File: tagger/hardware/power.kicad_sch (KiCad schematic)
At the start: 34 parts, among them J6 CHARGER, P1 USB, U12 TPS62A02DRL, U6 MAX77757JEFG420+T

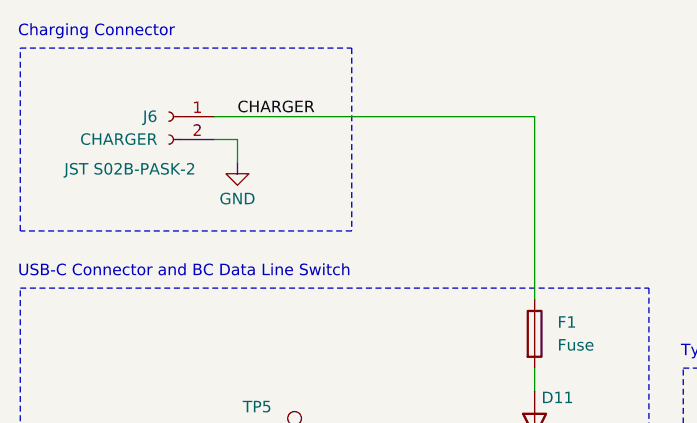
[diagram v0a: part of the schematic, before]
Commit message: chore(tagger): schematic reorganization
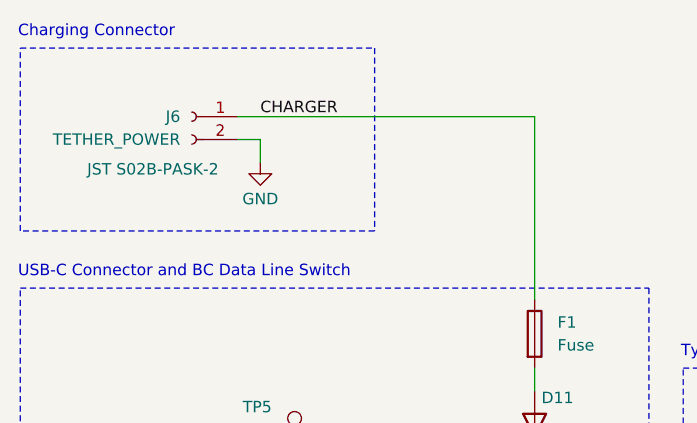
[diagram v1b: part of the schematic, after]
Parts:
- J6: value CHARGER -> TETHER_POWER
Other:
- moved on the sheet: J6
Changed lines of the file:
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@@
 	(rectangle
 		(start 17.78 20.32)
-		(end 54.61 40.64)
+		(end 57.15 40.64)
 		(stroke
 			(width 0)
@@
 	(wire
 		(pts
-			(xy 41.91 30.48) (xy 41.91 33.02)
+			(xy 44.45 30.48) (xy 44.45 33.02)
 		)
 		(stroke
@@
 	(wire
 		(pts
-			(xy 39.37 30.48) (xy 41.91 30.48)
+			(xy 41.91 30.48) (xy 44.45 30.48)
 		)
 		(stroke
@@
 	(wire
 		(pts
-			(xy 39.37 27.94) (xy 74.93 27.94)
+			(xy 41.91 27.94) (xy 74.93 27.94)
 		)
 		(stroke
@@
 	)
 	(label "CHARGER"
-		(at 41.91 27.94 0)
+		(at 44.45 27.94 0)
 		(effects
 			(font
@@
 	(symbol
 		(lib_id "Connector:Conn_01x02_Socket")
-		(at 34.29 27.94 0)
+		(at 36.83 27.94 0)
 		(mirror y)
 		(unit 1)
@@
 		(dnp no)
 		(property "Reference" "J6"
-			(at 33.02 27.9399 0)
+			(at 35.56 27.9399 0)
 			(effects
 				(font
@@
 			)
 		)
-		(property "Value" "CHARGER"
-			(at 33.02 30.4799 0)
+		(property "Value" "TETHER_POWER"
+			(at 35.56 30.4799 0)
 			(effects
 				(font
@@
 		)
 		(property "Footprint" ""
-			(at 34.29 27.94 0)
+			(at 36.83 27.94 0)
 			(effects
 				(font
@@
 		)
 		(property "Datasheet" "~"
-			(at 34.29 27.94 0)
+			(at 36.83 27.94 0)
 			(effects
 				(font
@@
 		)
 		(property "Description" "Generic connector, single row, 01x02, script generated"
-			(at 34.29 27.94 0)
+			(at 36.83 27.94 0)
 			(effects
 				(font
@@
 		)
 		(property "Conn" "JST S02B-PASK-2"
-			(at 29.972 33.782 0)
+			(at 32.512 33.782 0)
 			(effects
 				(font
@@
 	(symbol
 		(lib_id "power:GND")
-		(at 41.91 33.02 0)
+		(at 44.45 33.02 0)
 		(unit 1)
 		(exclude_from_sim no)
@@
 		(dnp no)
 		(property "Reference" "#PWR016"
-			(at 41.91 39.37 0)
+			(at 44.45 39.37 0)
 			(effects
 				(font
@@
 		)
 		(property "Value" "GND"
-			(at 41.91 37.084 0)
+			(at 44.45 37.084 0)
 			(effects
 				(font
@@
 		)
 		(property "Footprint" ""
-			(at 41.91 33.02 0)
+			(at 44.45 33.02 0)
 			(effects
 				(font
@@
 		)
 		(property "Datasheet" ""
-			(at 41.91 33.02 0)
+			(at 44.45 33.02 0)
 			(effects
 				(font
@@
 		)
 		(property "Description" "Power symbol creates a global label with name \"GND\" , ground"
-			(at 41.91 33.02 0)
+			(at 44.45 33.02 0)
 			(effects
 				(font
